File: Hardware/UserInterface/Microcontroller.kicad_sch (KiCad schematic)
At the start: 30 parts, among them J4001 USB_C_Receptacle_USB2.0_16P, J4002 TagConnect_SWD, SW4001 SW_Push, SW4002 SW_Push, U4001 W25Q64JVXGIQ, U4002 RP2040, Y4001 12M

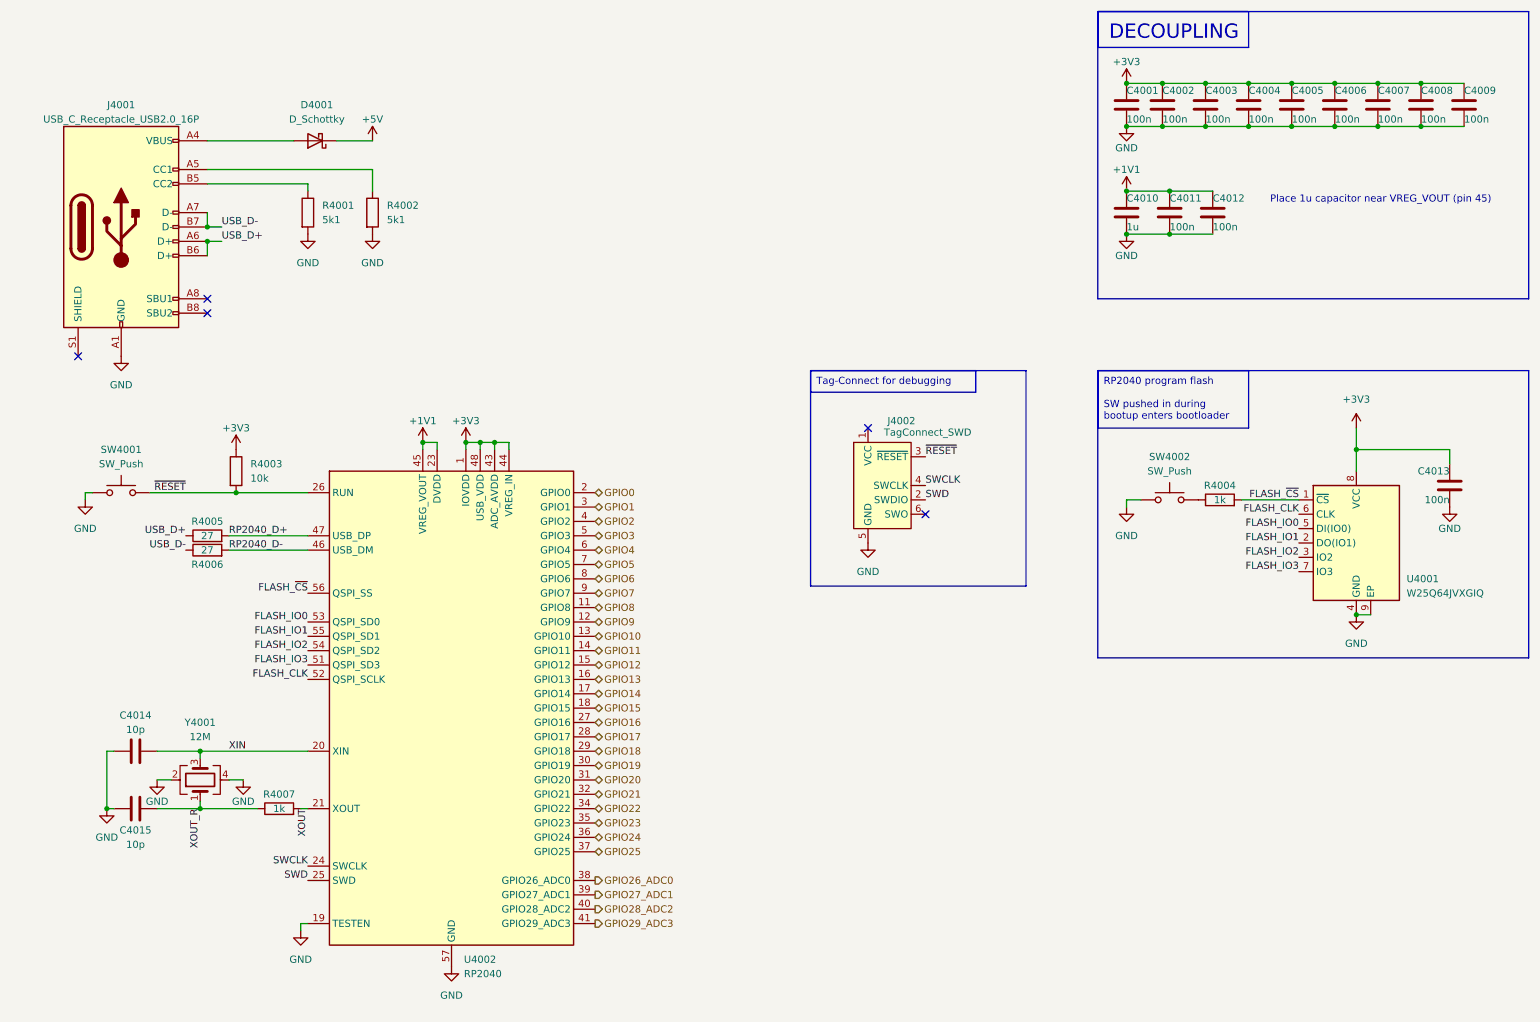
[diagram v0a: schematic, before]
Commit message: La in allt
Myyycket saker
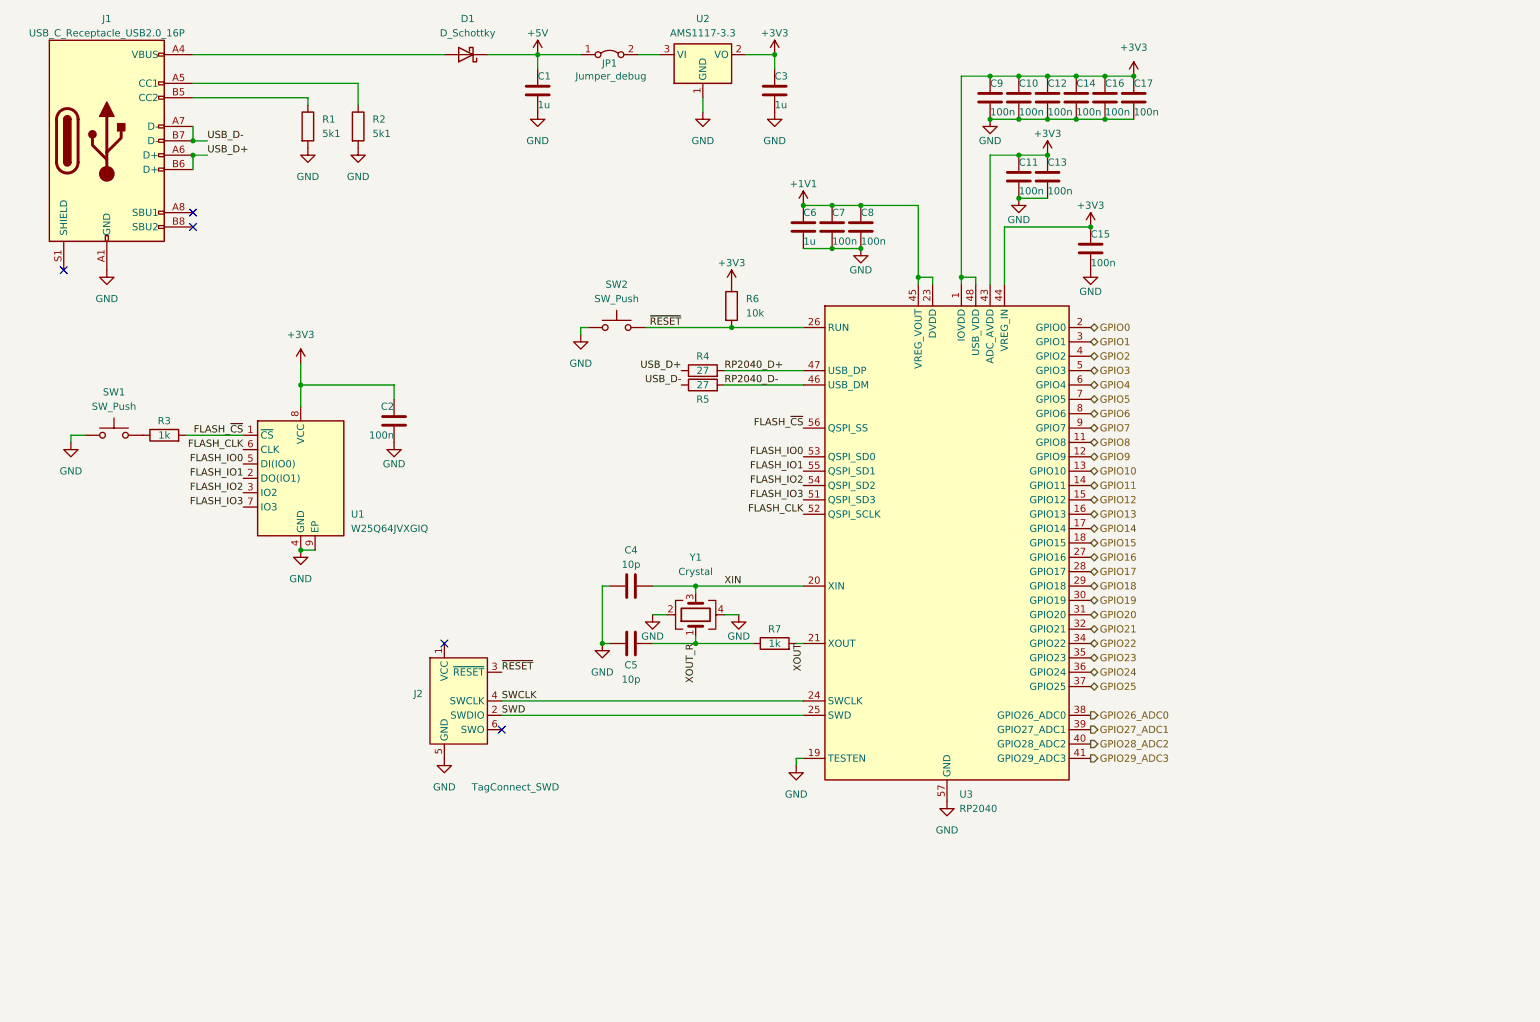
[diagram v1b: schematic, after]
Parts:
- removed C4001, C4002, C4003, C4004, C4005, C4006, C4007, C4008, C4009, C4011, C4012, C4013: 100n, Capacitor_SMD:C_0402_1005Metric, symbol Device:C
- removed C4010: 1u, Capacitor_SMD:C_0402_1005Metric, symbol Device:C
- removed C4014, C4015: 10p, Capacitor_SMD:C_0402_1005Metric, symbol Device:C
- removed D4001: D_Schottky, Diode_SMD:Nexperia_DSN1608-2_1.6x0.8mm, symbol Device:D_Schottky
- removed J4001: USB_C_Receptacle_USB2.0_16P, Connector_USB:USB_C_Receptacle_GCT_USB4105-xx-A_16P_TopMnt_Horizontal, symbol Connector:USB_C_Receptacle_USB2.0_16P
- removed J4002: TagConnect_SWD, Connector:Tag-Connect_TC2030-IDC-NL_2x03_P1.27mm_Vertical, symbol Connector:Conn_ARM_SWD_TagConnect_TC2030-NL
- removed R4001, R4002: 5k1, Resistor_SMD:R_0402_1005Metric, symbol Device:R
- removed R4003: 10k, Resistor_SMD:R_0402_1005Metric, symbol Device:R
- removed R4004, R4007: 1k, Resistor_SMD:R_0402_1005Metric, symbol Device:R
- removed R4005, R4006: 27, Resistor_SMD:R_0402_1005Metric, symbol Device:R
- removed SW4001, SW4002: SW_Push, Button_Switch_SMD:SW_Push_SPST_NO_Alps_SKRK, symbol Switch:SW_Push
- removed U4001: W25Q64JVXGIQ, Package_SON:WSON-8-1EP_4x4mm_P0.8mm_EP2.2x3mm, symbol Memory_Flash:W25Q32JVZP
- removed U4002: RP2040, Package_DFN_QFN:QFN-56-1EP_7x7mm_P0.4mm_EP3.2x3.2mm, symbol MCU_RaspberryPi:RP2040
- removed Y4001: 12M, Crystal:Crystal_SMD_Abracon_ABM3B-4Pin_5.0x3.2mm, symbol Device:Crystal_GND24
- added C1, C3, C6: 1u, Capacitor_SMD:C_0402_1005Metric, symbol Device:C
- added C10, C11, C12, C13, C14, C15, C16, C17, C2, C7, C8, C9: 100n, Capacitor_SMD:C_0402_1005Metric, symbol Device:C
- added C4, C5: 10p, Capacitor_SMD:C_0402_1005Metric, symbol Device:C
- added D1: D_Schottky, symbol Device:D_Schottky
- added J1: USB_C_Receptacle_USB2.0_16P, symbol Connector:USB_C_Receptacle_USB2.0_16P
- added J2: TagConnect_SWD, Connector:Tag-Connect_TC2030-IDC-NL_2x03_P1.27mm_Vertical, symbol Connector:Conn_ARM_SWD_TagConnect_TC2030-NL
- added JP1: Jumper_debug, symbol Jumper:Jumper_2_Bridged
- added R1, R2: 5k1, symbol Device:R
- added R3, R7: 1k, Resistor_SMD:R_0402_1005Metric, symbol Device:R
- added R4, R5: 27, Resistor_SMD:R_0402_1005Metric, symbol Device:R
- added R6: 10k, Resistor_SMD:R_0402_1005Metric, symbol Device:R
- added SW1, SW2: SW_Push, Button_Switch_SMD:SW_Push_SPST_NO_Alps_SKRK, symbol Switch:SW_Push
- added U1: W25Q64JVXGIQ, Package_SON:WSON-8-1EP_4x4mm_P0.8mm_EP2.2x3mm, symbol Memory_Flash:W25Q32JVZP
- added U2: AMS1117-3.3, Package_TO_SOT_SMD:SOT-223-3_TabPin2, symbol Regulator_Linear:AMS1117-3.3
- added U3: RP2040, Package_DFN_QFN:QFN-56-1EP_7x7mm_P0.4mm_EP3.2x3.2mm, symbol MCU_RaspberryPi:RP2040
- added Y1: Crystal, Crystal:Crystal_SMD_Abracon_ABM3B-4Pin_5.0x3.2mm, symbol Device:Crystal_GND24
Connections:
- net +1V1: now also C6.1, C7.1, C8.1, U3.23 (DVDD), U3.45 (VREG_VOUT), U3.50 (DVDD)
- net +3V3: now also C10.1, C11.1, C12.1, C13.1, C14.1, C15.1, C16.1, C17.1, C2.1, C3.1, C9.1, R6.1, U1.8 (VCC), U2.2 (VO), U3.1 (IOVDD), U3.10 (IOVDD), U3.22 (IOVDD), U3.33 (IOVDD), U3.42 (IOVDD), U3.43 (ADC_AVDD), U3.44 (VREG_IN), U3.48 (USB_VDD), U3.49 (IOVDD)
- net +5V: now also C1.1, D1.1 (K), JP1.1 (A)
- net FLASH_CLK: now also U1.6 (CLK), U3.52 (QSPI_SCLK)
- net FLASH_IO0: now also U1.5 (DI(IO0)), U3.53 (QSPI_SD0)
- net FLASH_IO1: now also U1.2 (DO(IO1)), U3.55 (QSPI_SD1)
- net FLASH_IO2: now also U1.3 (IO2), U3.54 (QSPI_SD2)
- net FLASH_IO3: now also U1.7 (IO3), U3.51 (QSPI_SD3)
- net FLASH_~{CS}: now also R3.2, U1.1 (~{CS}), U3.56 (QSPI_SS)
- net GND: now also C1.2, C10.2, C11.2, C12.2, C13.2, C14.2, C15.2, C16.2, C17.2, C2.2, C3.2, C4.1, C5.1, C6.2, C7.2, C8.2, C9.2, J1.A1 (GND), J1.A12 (GND), J1.B1 (GND), J1.B12 (GND), J2.5 (GND), R1.2, R2.2, SW1.1, SW2.2, U1.4 (GND), U1.9 (EP), U2.1 (GND), U3.19 (TESTEN), U3.57 (GND), Y1.2, Y1.4
- net GPIO0: now also U3.2 (GPIO0)
- net GPIO1: now also U3.3 (GPIO1)
- net GPIO10: now also U3.13 (GPIO10)
- net GPIO11: now also U3.14 (GPIO11)
- net GPIO12: now also U3.15 (GPIO12)
- net GPIO13: now also U3.16 (GPIO13)
- net GPIO14: now also U3.17 (GPIO14)
- net GPIO15: now also U3.18 (GPIO15)
- net GPIO16: now also U3.27 (GPIO16)
- net GPIO17: now also U3.28 (GPIO17)
- net GPIO18: now also U3.29 (GPIO18)
- net GPIO19: now also U3.30 (GPIO19)
- net GPIO2: now also U3.4 (GPIO2)
- net GPIO20: now also U3.31 (GPIO20)
- net GPIO21: now also U3.32 (GPIO21)
- net GPIO22: now also U3.34 (GPIO22)
- net GPIO23: now also U3.35 (GPIO23)
- net GPIO24: now also U3.36 (GPIO24)
- net GPIO25: now also U3.37 (GPIO25)
- net GPIO26_ADC0: now also U3.38 (GPIO26_ADC0)
- net GPIO27_ADC1: now also U3.39 (GPIO27_ADC1)
- net GPIO28_ADC2: now also U3.40 (GPIO28_ADC2)
- net GPIO29_ADC3: now also U3.41 (GPIO29_ADC3)
- net GPIO3: now also U3.5 (GPIO3)
- net GPIO4: now also U3.6 (GPIO4)
- net GPIO5: now also U3.7 (GPIO5)
- net GPIO6: now also U3.8 (GPIO6)
- net GPIO7: now also U3.9 (GPIO7)
- net GPIO8: now also U3.11 (GPIO8)
- net GPIO9: now also U3.12 (GPIO9)
- net RP2040_D+: now also R4.2, U3.47 (USB_DP)
- net RP2040_D-: now also R5.2, U3.46 (USB_DM)
- net SWCLK: now also J2.4 (SWCLK), U3.24 (SWCLK)
- net SWD: now also J2.2 (SWDIO), U3.25 (SWD)
- net USB_D+: now also J1.A6 (D+), J1.B6 (D+), R4.1
- net USB_D-: now also J1.A7 (D-), J1.B7 (D-), R5.1
- net XIN: now also C4.2, U3.20 (XIN), Y1.3
- net XOUT: now also R7.2, U3.21 (XOUT)
- net XOUT_R: now also C5.2, R7.1, Y1.1
- net ~{RESET}: now also J2.3 (~{RESET}), R6.2, SW2.1, U3.26 (RUN)
- new net: J1.B5 (CC2), R1.1
- new net: J1.A5 (CC1), R2.1
- new net: R3.1, SW1.2
- new net: JP1.2 (B), U2.3 (VI)
- new net: D1.2 (A), J1.A4 (VBUS), J1.A9 (VBUS), J1.B4 (VBUS), J1.B9 (VBUS)
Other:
- note removed: "Place 1u capacitor near VREG_VOUT (pin 45)"
- company: Chalmers EENX16-VT24-27 -> (none)

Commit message: User interface fix
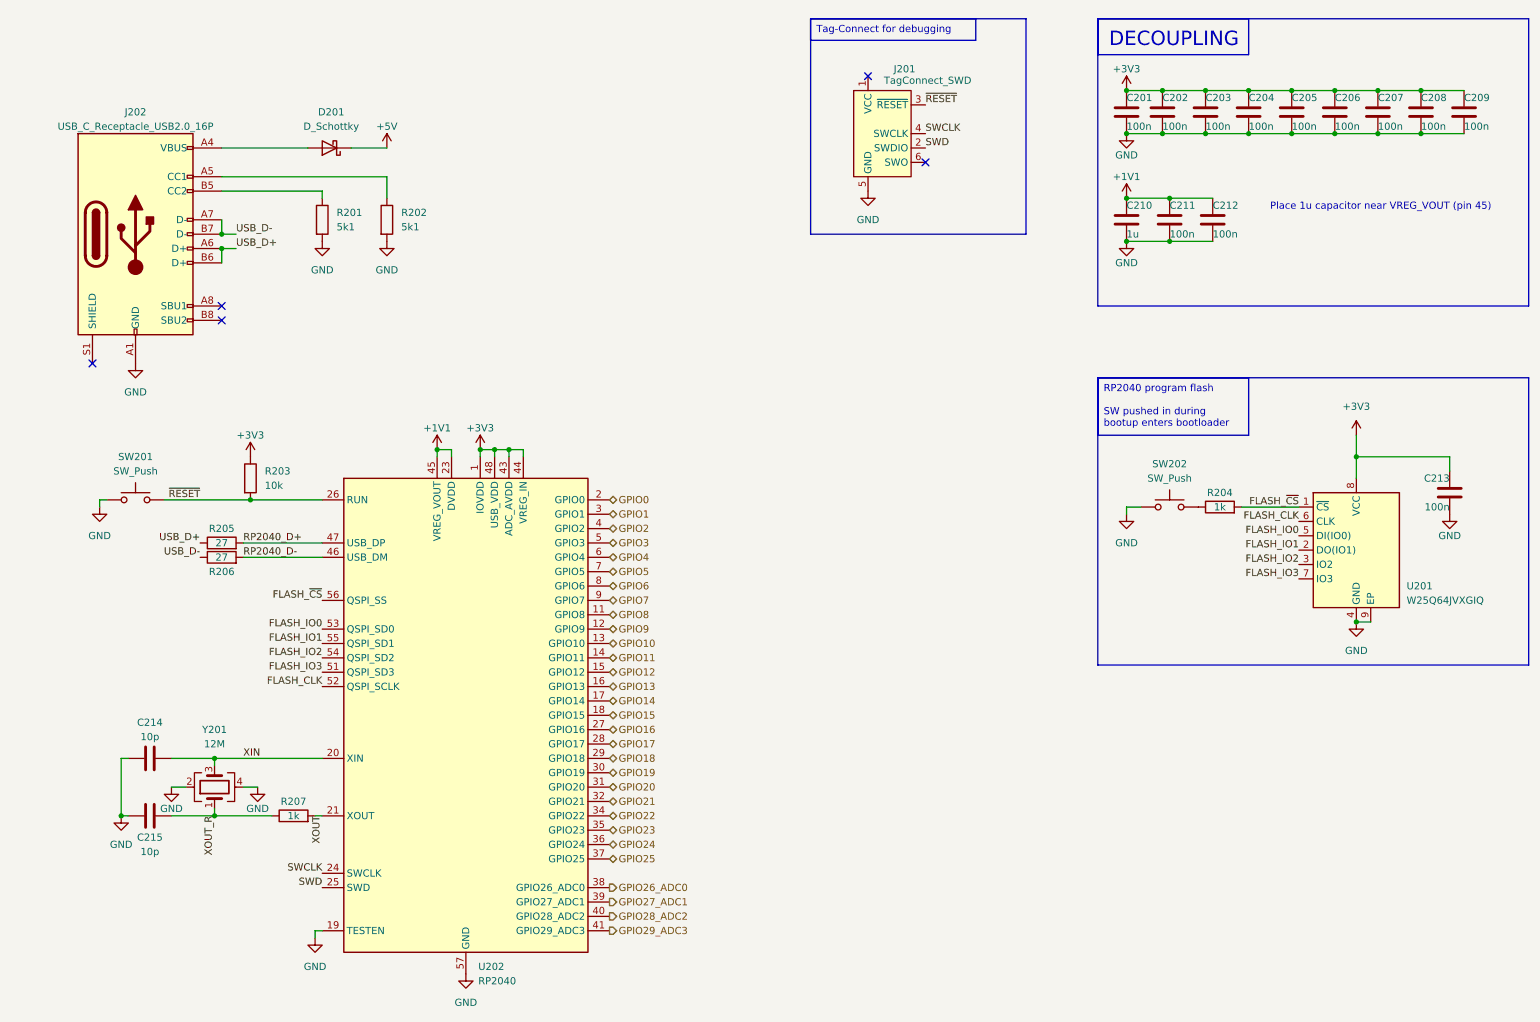
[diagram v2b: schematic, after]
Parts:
- removed C1, C3, C6: 1u, Capacitor_SMD:C_0402_1005Metric, symbol Device:C
- removed C10, C11, C12, C13, C14, C15, C16, C17, C2, C7, C8, C9: 100n, Capacitor_SMD:C_0402_1005Metric, symbol Device:C
- removed C4, C5: 10p, Capacitor_SMD:C_0402_1005Metric, symbol Device:C
- removed D1: D_Schottky, symbol Device:D_Schottky
- removed J1: USB_C_Receptacle_USB2.0_16P, symbol Connector:USB_C_Receptacle_USB2.0_16P
- removed J2: TagConnect_SWD, Connector:Tag-Connect_TC2030-IDC-NL_2x03_P1.27mm_Vertical, symbol Connector:Conn_ARM_SWD_TagConnect_TC2030-NL
- removed JP1: Jumper_debug, symbol Jumper:Jumper_2_Bridged
- removed R1, R2: 5k1, symbol Device:R
- removed R3, R7: 1k, Resistor_SMD:R_0402_1005Metric, symbol Device:R
- removed R4, R5: 27, Resistor_SMD:R_0402_1005Metric, symbol Device:R
- removed R6: 10k, Resistor_SMD:R_0402_1005Metric, symbol Device:R
- removed SW1, SW2: SW_Push, Button_Switch_SMD:SW_Push_SPST_NO_Alps_SKRK, symbol Switch:SW_Push
- removed U1: W25Q64JVXGIQ, Package_SON:WSON-8-1EP_4x4mm_P0.8mm_EP2.2x3mm, symbol Memory_Flash:W25Q32JVZP
- removed U2: AMS1117-3.3, Package_TO_SOT_SMD:SOT-223-3_TabPin2, symbol Regulator_Linear:AMS1117-3.3
- removed U3: RP2040, Package_DFN_QFN:QFN-56-1EP_7x7mm_P0.4mm_EP3.2x3.2mm, symbol MCU_RaspberryPi:RP2040
- removed Y1: Crystal, Crystal:Crystal_SMD_Abracon_ABM3B-4Pin_5.0x3.2mm, symbol Device:Crystal_GND24
- added C201, C202, C203, C204, C205, C206, C207, C208, C209, C211, C212, C213: 100n, Capacitor_SMD:C_0402_1005Metric, symbol Device:C
- added C210: 1u, Capacitor_SMD:C_0402_1005Metric, symbol Device:C
- added C214, C215: 10p, Capacitor_SMD:C_0402_1005Metric, symbol Device:C
- added D201: D_Schottky, Diode_SMD:Nexperia_DSN1608-2_1.6x0.8mm, symbol Device:D_Schottky
- added J201: TagConnect_SWD, Connector:Tag-Connect_TC2030-IDC-NL_2x03_P1.27mm_Vertical, symbol Connector:Conn_ARM_SWD_TagConnect_TC2030-NL
- added J202: USB_C_Receptacle_USB2.0_16P, Connector_USB:USB_C_Receptacle_GCT_USB4105-xx-A_16P_TopMnt_Horizontal, symbol Connector:USB_C_Receptacle_USB2.0_16P
- added R201, R202: 5k1, Resistor_SMD:R_0402_1005Metric, symbol Device:R
- added R203: 10k, Resistor_SMD:R_0402_1005Metric, symbol Device:R
- added R204, R207: 1k, Resistor_SMD:R_0402_1005Metric, symbol Device:R
- added R205, R206: 27, Resistor_SMD:R_0402_1005Metric, symbol Device:R
- added SW201, SW202: SW_Push, Button_Switch_SMD:SW_Push_SPST_NO_Alps_SKRK, symbol Switch:SW_Push
- added U201: W25Q64JVXGIQ, Package_SON:WSON-8-1EP_4x4mm_P0.8mm_EP2.2x3mm, symbol Memory_Flash:W25Q32JVZP
- added U202: RP2040, Package_DFN_QFN:QFN-56-1EP_7x7mm_P0.4mm_EP3.2x3.2mm, symbol MCU_RaspberryPi:RP2040
- added Y201: 12M, Crystal:Crystal_SMD_Abracon_ABM3B-4Pin_5.0x3.2mm, symbol Device:Crystal_GND24
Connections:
- net +1V1: now also C210.1, C211.1, C212.1, U202.23 (DVDD), U202.45 (VREG_VOUT), U202.50 (DVDD)
- net +3V3: now also C201.1, C202.1, C203.1, C204.1, C205.1, C206.1, C207.1, C208.1, C209.1, C213.1, R203.1, U201.8 (VCC), U202.1 (IOVDD), U202.10 (IOVDD), U202.22 (IOVDD), U202.33 (IOVDD), U202.42 (IOVDD), U202.43 (ADC_AVDD), U202.44 (VREG_IN), U202.48 (USB_VDD), U202.49 (IOVDD)
- net +5V: now also D201.1 (K)
- net FLASH_CLK: now also U201.6 (CLK), U202.52 (QSPI_SCLK)
- net FLASH_IO0: now also U201.5 (DI(IO0)), U202.53 (QSPI_SD0)
- net FLASH_IO1: now also U201.2 (DO(IO1)), U202.55 (QSPI_SD1)
- net FLASH_IO2: now also U201.3 (IO2), U202.54 (QSPI_SD2)
- net FLASH_IO3: now also U201.7 (IO3), U202.51 (QSPI_SD3)
- net FLASH_~{CS}: now also R204.2, U201.1 (~{CS}), U202.56 (QSPI_SS)
- net GND: now also C201.2, C202.2, C203.2, C204.2, C205.2, C206.2, C207.2, C208.2, C209.2, C210.2, C211.2, C212.2, C213.2, C214.1, C215.1, J201.5 (GND), J202.A1 (GND), J202.A12 (GND), J202.B1 (GND), J202.B12 (GND), R201.2, R202.2, SW201.2, SW202.1, U201.4 (GND), U201.9 (EP), U202.19 (TESTEN), U202.57 (GND), Y201.2, Y201.4
- net GPIO0: now also U202.2 (GPIO0)
- net GPIO1: now also U202.3 (GPIO1)
- net GPIO10: now also U202.13 (GPIO10)
- net GPIO11: now also U202.14 (GPIO11)
- net GPIO12: now also U202.15 (GPIO12)
- net GPIO13: now also U202.16 (GPIO13)
- net GPIO14: now also U202.17 (GPIO14)
- net GPIO15: now also U202.18 (GPIO15)
- net GPIO16: now also U202.27 (GPIO16)
- net GPIO17: now also U202.28 (GPIO17)
- net GPIO18: now also U202.29 (GPIO18)
- net GPIO19: now also U202.30 (GPIO19)
- net GPIO2: now also U202.4 (GPIO2)
- net GPIO20: now also U202.31 (GPIO20)
- net GPIO21: now also U202.32 (GPIO21)
- net GPIO22: now also U202.34 (GPIO22)
- net GPIO23: now also U202.35 (GPIO23)
- net GPIO24: now also U202.36 (GPIO24)
- net GPIO25: now also U202.37 (GPIO25)
- net GPIO26_ADC0: now also U202.38 (GPIO26_ADC0)
- net GPIO27_ADC1: now also U202.39 (GPIO27_ADC1)
- net GPIO28_ADC2: now also U202.40 (GPIO28_ADC2)
- net GPIO29_ADC3: now also U202.41 (GPIO29_ADC3)
- net GPIO3: now also U202.5 (GPIO3)
- net GPIO4: now also U202.6 (GPIO4)
- net GPIO5: now also U202.7 (GPIO5)
- net GPIO6: now also U202.8 (GPIO6)
- net GPIO7: now also U202.9 (GPIO7)
- net GPIO8: now also U202.11 (GPIO8)
- net GPIO9: now also U202.12 (GPIO9)
- net RP2040_D+: now also R205.2, U202.47 (USB_DP)
- net RP2040_D-: now also R206.2, U202.46 (USB_DM)
- net SWCLK: now also J201.4 (SWCLK), U202.24 (SWCLK)
- net SWD: now also J201.2 (SWDIO), U202.25 (SWD)
- net USB_D+: now also J202.A6 (D+), J202.B6 (D+), R205.1
- net USB_D-: now also J202.A7 (D-), J202.B7 (D-), R206.1
- net XIN: now also C214.2, U202.20 (XIN), Y201.3
- net XOUT: now also R207.2, U202.21 (XOUT)
- net XOUT_R: now also C215.2, R207.1, Y201.1
- net ~{RESET}: now also J201.3 (~{RESET}), R203.2, SW201.1, U202.26 (RUN)
- new net: J202.B5 (CC2), R201.1
- new net: R204.1, SW202.2
- new net: D201.2 (A), J202.A4 (VBUS), J202.A9 (VBUS), J202.B4 (VBUS), J202.B9 (VBUS)
- new net: J202.A5 (CC1), R202.1
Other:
- note added: "Place 1u capacitor near VREG_VOUT (pin 45)"

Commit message: Changes and fixes
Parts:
- Y201: footprint Crystal:Crystal_SMD_Abracon_ABM3B-4Pin_5.0x3.2mm -> Crystal:Crystal_SMD_2520-4Pin_2.5x2.0mm; mouser 815-ABM3B1210B1UT -> 520-120-10-36Q-AEST
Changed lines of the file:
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@@
 			)
 		)
-		(property "Footprint" "Crystal:Crystal_SMD_Abracon_ABM3B-4Pin_5.0x3.2mm"
+		(property "Footprint" "Crystal:Crystal_SMD_2520-4Pin_2.5x2.0mm"
 			(at 46.99 149.86 0)
 			(effects
@@
 			)
 		)
-		(property "Datasheet" "https://eu.mouser.com/datasheet/2/3/abm3b-1774998.pdf"
+		(property "Datasheet" "https://www.mouser.se/datasheet/2/122/ECX_2236Q-938171.pdf"
 			(at 46.99 149.86 0)
 			(effects
@@
 			)
 		)
-		(property "mouser" "815-ABM3B1210B1UT"
+		(property "mouser" "520-120-10-36Q-AEST"
 			(at 46.99 149.86 0)
 			(effects
